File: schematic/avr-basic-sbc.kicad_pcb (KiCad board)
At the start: 2 copper layers, 94 x 55 mm, 43 parts, among them J1 DC-005 Power Jack, J2 PS/2 keyboard port, J3 Power output header, J4 RCA Video Jack, J5 USBasp header, J6 Port A, J7 Port B, J8 Port C, J9 Port D, U1 L7805, U2 ATmega1284P-P, U3 25LC640, Y1 16 MHz

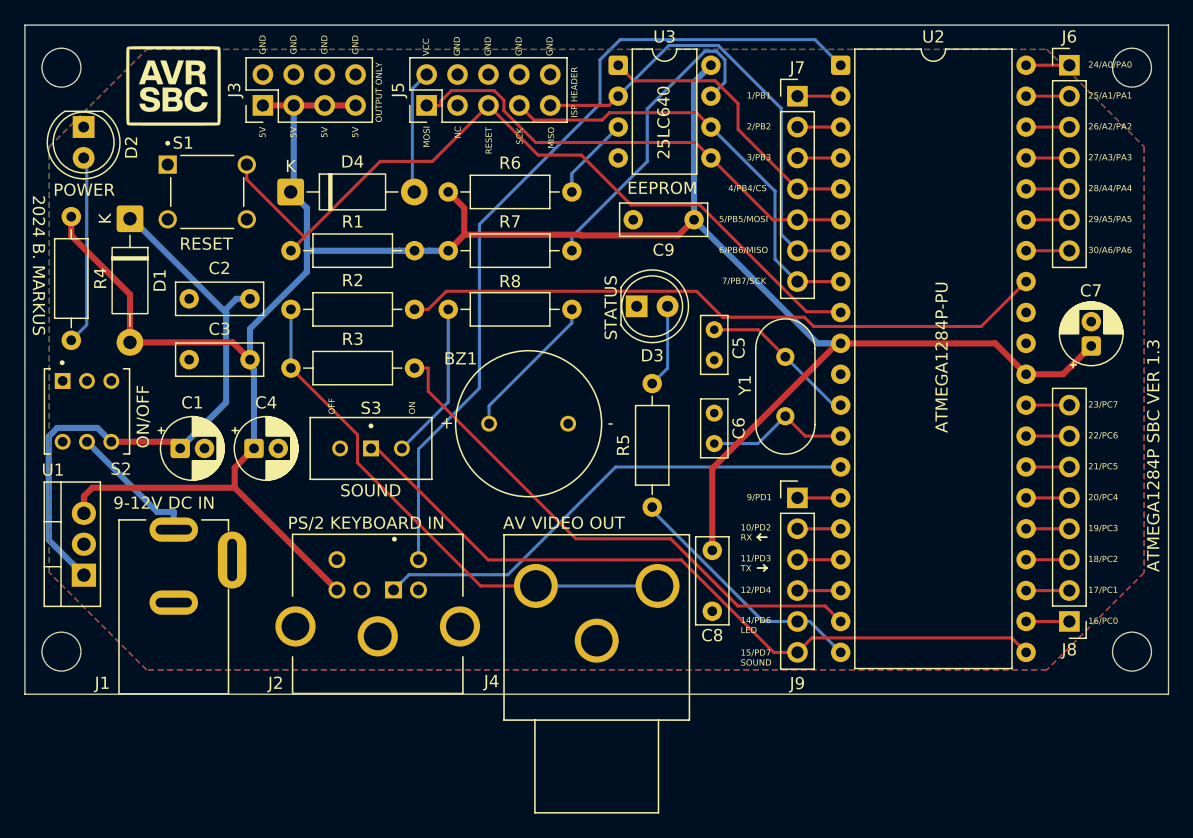
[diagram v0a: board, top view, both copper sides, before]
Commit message: PCB reverted to release version v1.2
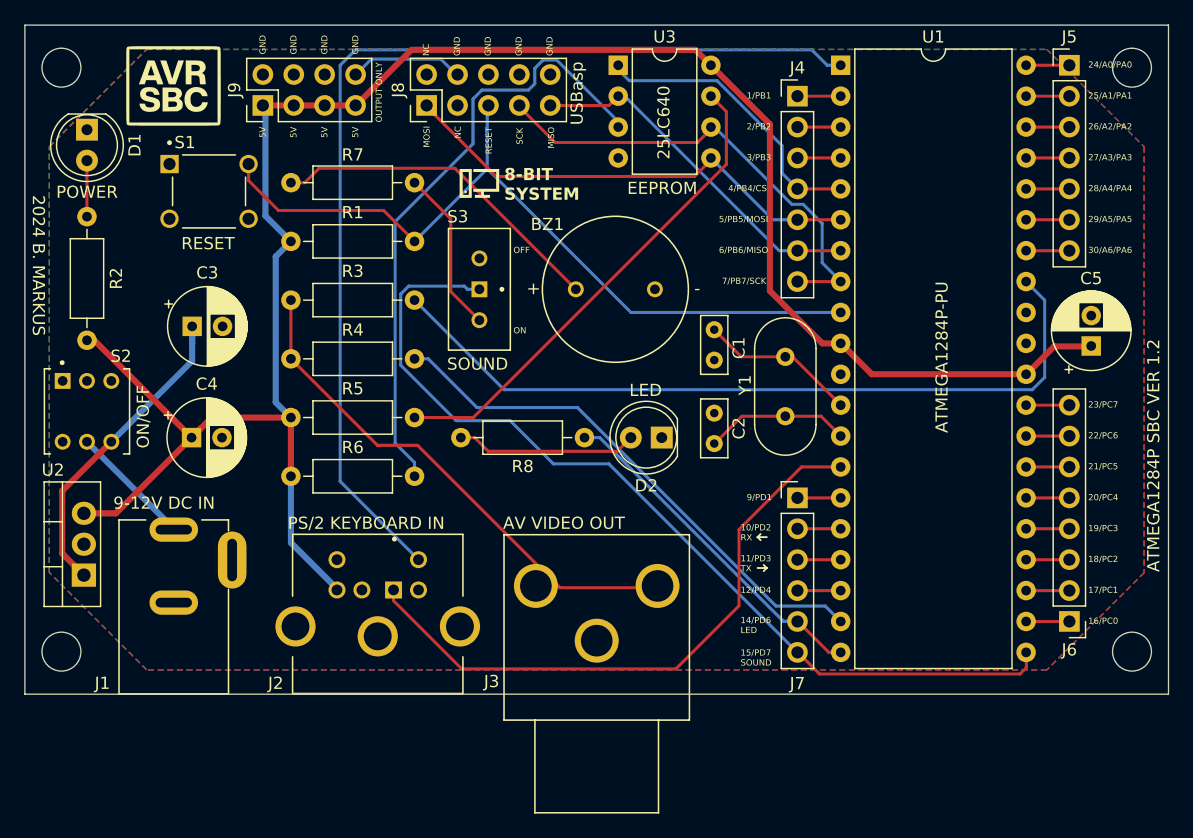
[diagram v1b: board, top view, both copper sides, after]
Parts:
- removed the C1 at (12.8, 34.8)
- removed the C2 at (13.5, 22.5)
- removed C8, C9: 0.1uF, StockLib:C_100nF_L7.0mm_W2.5mm_P5.00mm
- removed the D1 at (8.64, 15.9)
- removed D4: 1N5819, Diode_THT:D_DO-41_SOD81_P10.16mm_Horizontal
- added GRAPHICS2: LOGO, LOGO, F.Cu at (37.4, 13.0)
- C3: value 0.1uF -> 0.33uF; footprint StockLib:C_100nF_L7.0mm_W2.5mm_P5.00mm -> Capacitor_THT:CP_Radial_D6.3mm_P2.50mm
- C4: value 10uF -> 0.1uF; footprint Capacitor_THT:CP_Radial_D5.0mm_P2.00mm -> Capacitor_THT:CP_Radial_D6.3mm_P2.50mm
- C5: renamed from C7; footprint Capacitor_THT:CP_Radial_D5.0mm_P2.00mm -> Capacitor_THT:CP_Radial_D6.3mm_P2.50mm
- moved R6 26.7 mm to (21.9, 37.1)
- moved R5 18.9 mm to (21.9, 32.3)
- moved S3 15.8 mm to (37.4, 21.7), turned to 90 degrees
- moved BZ1 13.2 mm to (48.5, 21.7)
- moved D2 11.0 mm to (52.3, 33.9), turned to 180 degrees
- moved R7 10.8 mm to (32.0, 13.0), turned to 180 degrees
- moved R8 7.98 mm to (46.0, 33.9), turned to 180 degrees
- moved C4 5.21 mm to (13.7, 33.9)
- moved C3 2.75 mm to (13.7, 24.8)
- moved R2 1.29 mm to (5.10, 25.9)
- moved R1 0.76 mm to (21.9, 17.8)
- moved R4 0.76 mm to (21.9, 27.4)
- moved R3 0.76 mm to (21.9, 22.6)
- moved D1 0.35 mm to (5.10, 8.60)
- moved S1 0.15 mm to (15.1, 13.7)
- renumbered C5 to C1, C6 to C2, D2 to D1, D3 to D2, J4 to J3, J7 to J4, J6 to J5, J8 to J6, J9 to J7, J5 to J8, J3 to J9, R4 to R2, R2 to R3, R3 to R4, R7 to R5, R8 to R7, R5 to R8, U2 to U1, U1 to U2
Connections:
- C3 pad 1: GND -> /POWER IN 2
- C3 pad 2: +5V -> GND
- D1 pad 2: Net-(D2-A) (its old number) -> Net-(D1-A)
- J8 pad 2: Net-(D4-A) -> unconnected-(J8-Pin_2-Pad2)
- R1 pad 1: RESET -> +5V
- R1 pad 2: +5V -> RESET
- R2 pad 1: Net-(D2-A) (its old number) -> +5V
- R2 pad 2: +5V -> Net-(D1-A)
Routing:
- net Net-(U3-~{WP}): track 6.91 -> 51.2 mm
- net +5V: track 201.9 -> 166.4 mm
- net /POWER IN 2: track 51.1 -> 27.0 mm
- net Clock: track 68.6 -> 85.5 mm
- net Net-(BZ1-+): track 12.2 -> 28.0 mm
- net Net-(D2-A) (its old number): track 15.6 -> 0.00 mm
- net Net-(J7-Pin_6): track 61.8 -> 76.1 mm
- net Net-(U3-~{HOLD}): track 26.3 -> 40.4 mm
- net Net-(D4-A): track 10.2 -> 0.00 mm
- net Video: track 53.6 -> 63.8 mm
- net Data: track 40.9 -> 50.5 mm
- net MISO: track 39.0 -> 29.6 mm
- net GND: track 0.00 -> 9.30 mm
- net Net-(D2-A): track 6.87 -> 14.9 mm
- net Net-(J7-Pin_5): track 20.9 -> 28.4 mm
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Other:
- board text added: "8-BIT SYSTEM"
- board text added: "ATMEGA1284P SBC VER 1.2"
- board text added: "LED"
- board text added: "USBasp"
- board text removed: "ATMEGA1284P SBC VER 1.3"
- board text removed: "ISP HEADER"
- board text removed: "STATUS"
- board text removed: "VCC"
